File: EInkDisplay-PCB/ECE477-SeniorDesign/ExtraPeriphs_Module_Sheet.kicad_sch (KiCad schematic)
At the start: 6 parts, among them J1 SD_Card_Device

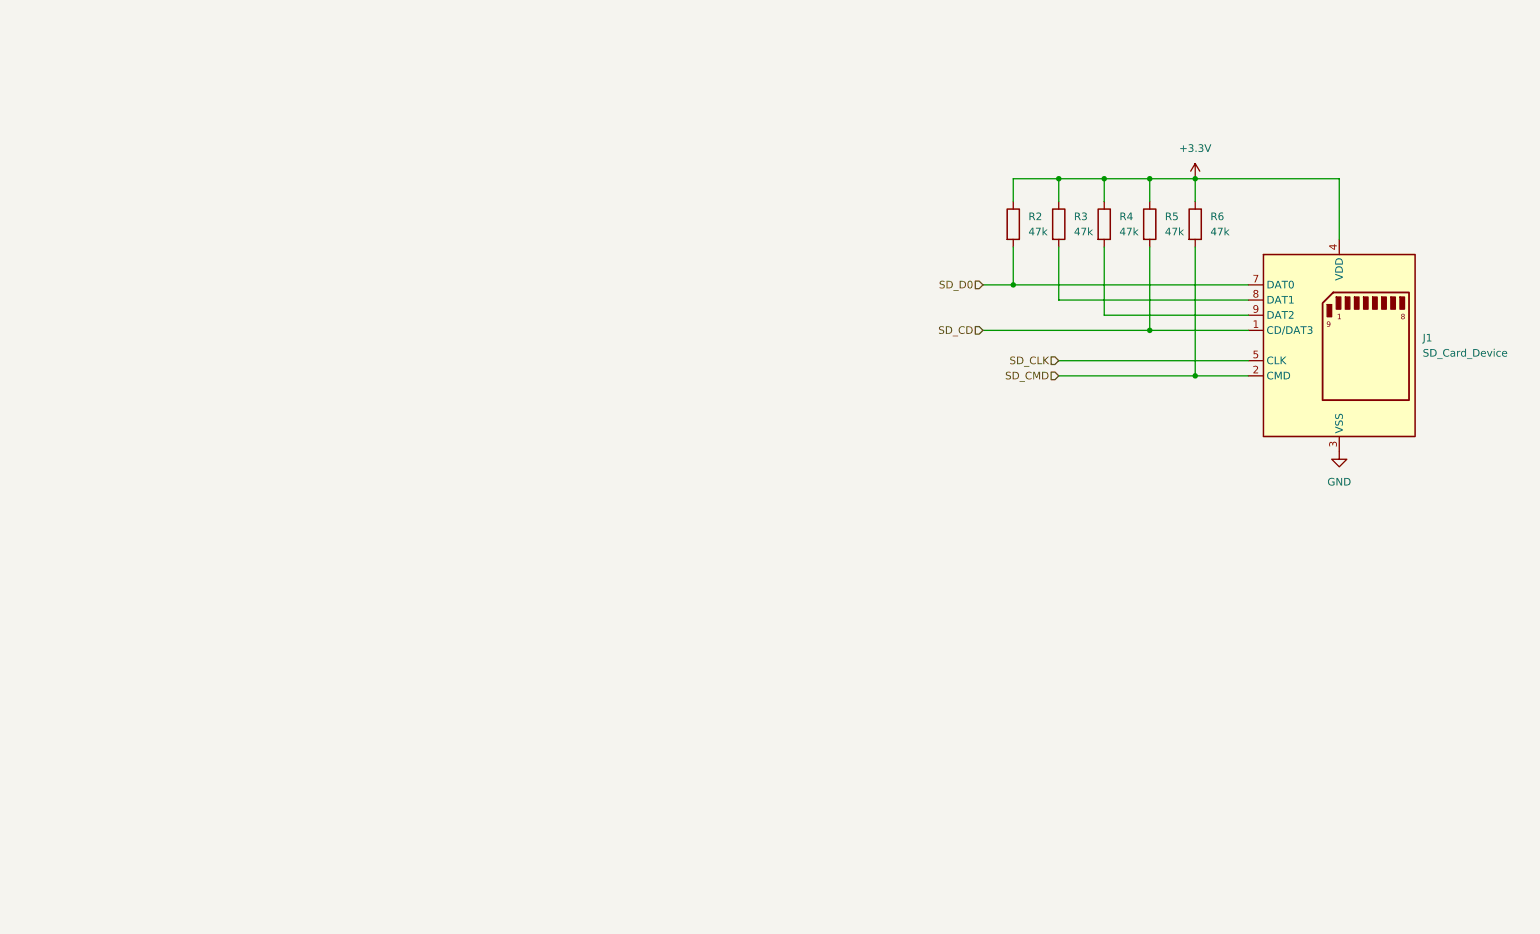
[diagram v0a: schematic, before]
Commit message: push
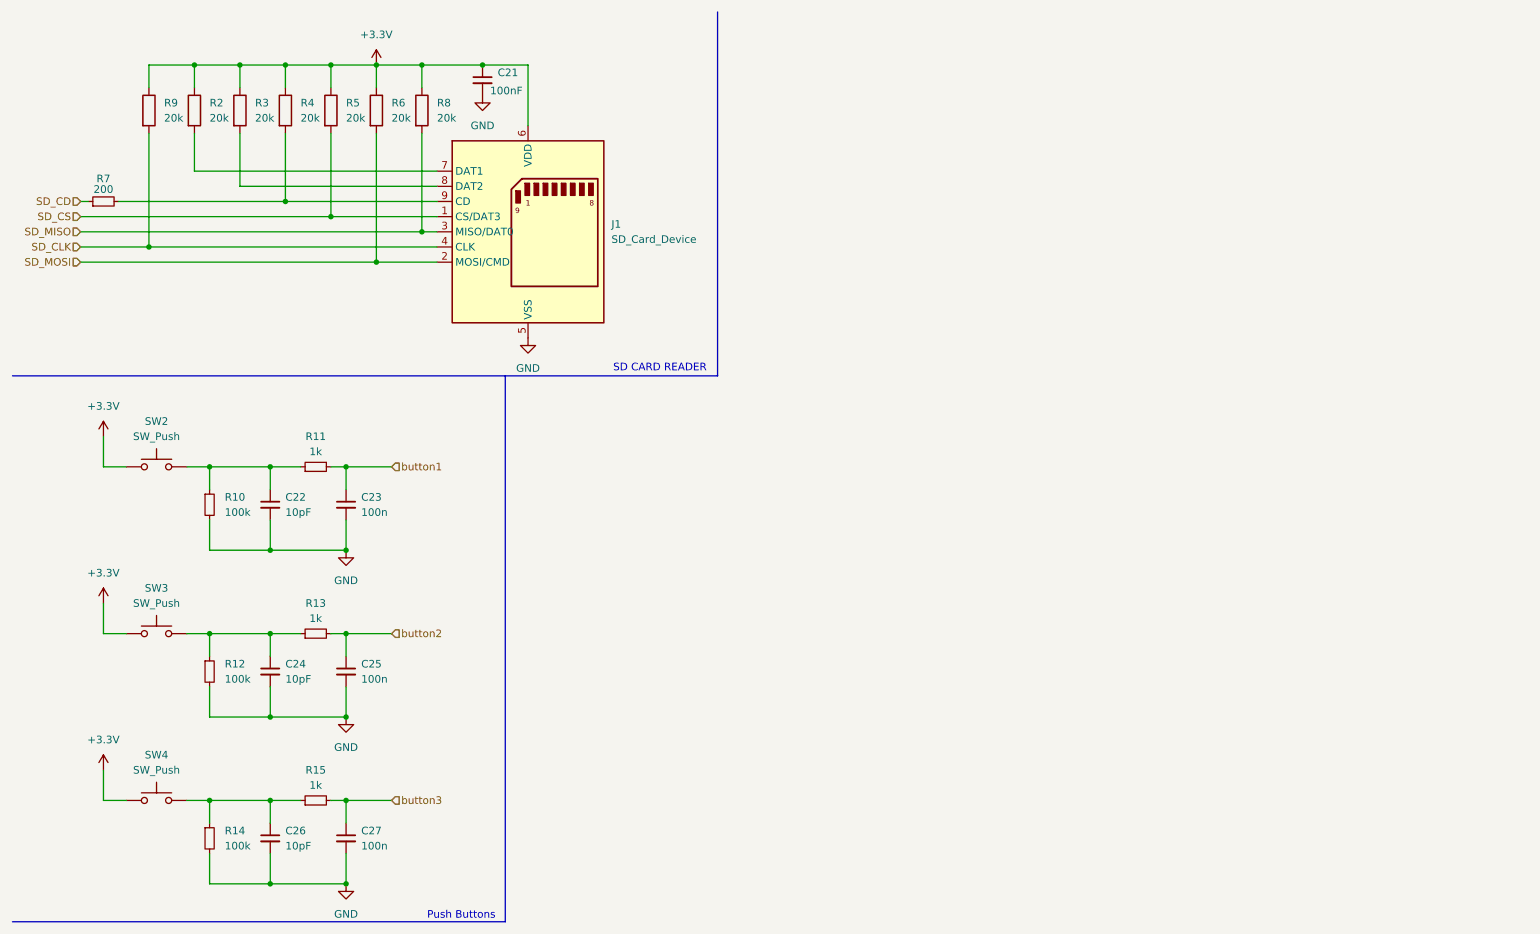
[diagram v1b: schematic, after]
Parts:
- added C21: 100nF, symbol Device:C_Small
- added C22, C24, C26: 10pF, symbol Device:C_Small
- added C23, C25, C27: 100n, symbol Device:C_Small
- added R10, R12, R14: 100k, symbol Device:R_Small
- added R11, R13, R15: 1k, symbol Device:R_Small
- added R7: 200, symbol Device:R_Small
- added R8, R9: 20k, symbol Device:R
- added SW2, SW3, SW4: SW_Push, symbol Switch:SW_Push
- R2, R3, R4, R5, R6: value 47k -> 20k
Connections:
- net +3.3V: now also J1.6 (VDD), C21.1, R8.1, R9.1, SW2.1, SW3.1, SW4.1; no longer J1.4 (VDD)
- net GND: now also J1.5 (VSS), C21.2, C22.2, C23.2, C24.2, C25.2, C26.2, C27.2, R10.2, R12.2, R14.2; no longer J1.3 (VSS), J1.6 (VSS)
- net SD_CD: now also R7.1; no longer J1.1 (CD/DAT3), R5.2
- net SD_CLK: now also J1.4 (CLK), R9.2; no longer J1.5 (CLK)
- net at J1.9 (CD), R4.2: now also R7.2
- net SD_CMD renamed SD_MOSI
- net SD_D0: no longer names the net of J1.7 (DAT1), R2.2
- new net: C24.1, R12.1, R13.1, SW3.2
- new net: C26.1, R14.1, R15.1, SW4.2
- new net: C22.1, R10.1, R11.1, SW2.2
- new net SD_CS: J1.1 (CS/DAT3), R5.2
- new net SD_MISO: J1.3 (MISO/DAT0), R8.2
- new net button1: C23.1, R11.2
- new net button2: C25.1, R13.2
- new net button3: C27.1, R15.2
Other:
- note added: "Push Buttons"
- note added: "SD CARD READER"
- moved on the sheet: R2, R3, R4, R5, R6
